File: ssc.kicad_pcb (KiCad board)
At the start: 4 copper layers, 98.8 x 85.1 mm, 25 parts, among them J1 IRQ ENABLE, J2 RS-232 OUT, P1 A2Bus, U1 74HCT245, U2 28C256, U3 1.8432M, U4 SSCGLU, U5 W65C51NxP, U6 MAX3232, U7 MAX3232

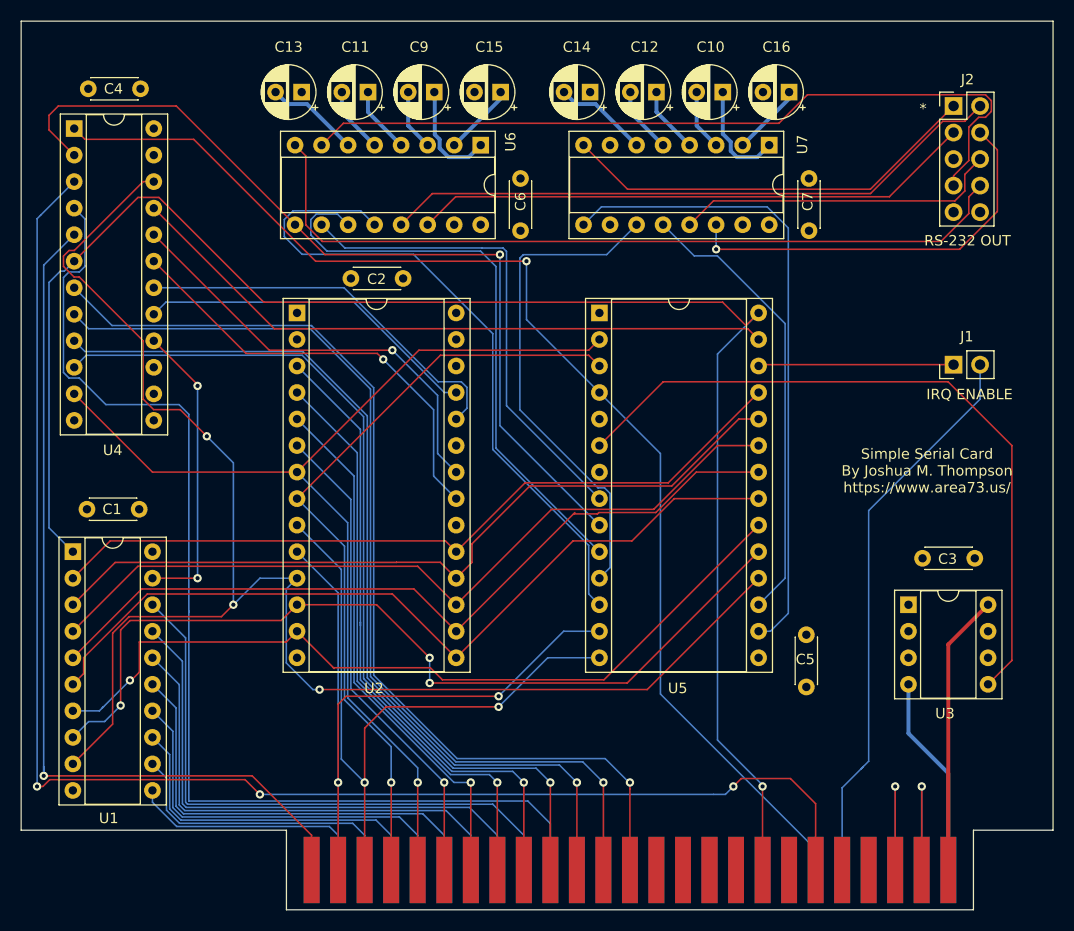
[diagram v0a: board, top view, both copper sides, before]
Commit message: Checkpoint.
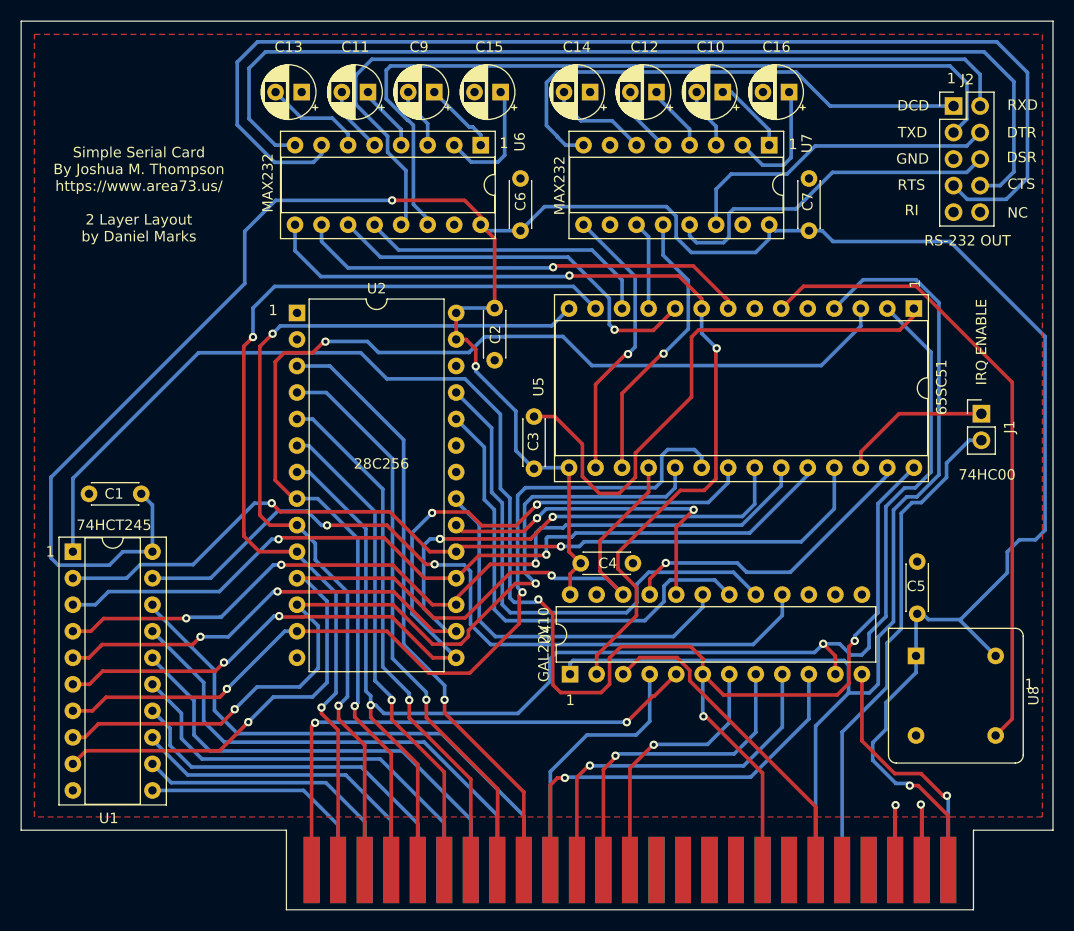
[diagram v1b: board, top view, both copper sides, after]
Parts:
- removed U3: 1.8432M, Package_DIP:DIP-8_W7.62mm_Socket
- added U8: 1.8432M, Oscillator:Oscillator_DIP-8, F.Cu at (187.3, 102.7)
- U1: value 74HCT245 -> 74LS245
- U2: value 28C256 -> 27C256; footprint Package_DIP:DIP-28_W15.24mm_Socket -> Package_DIP:DIP-28_W15.24mm
- U4: footprint Package_DIP:DIP-24_W7.62mm_Socket -> Package_DIP:DIP-24_W7.62mm
- moved U4 70.6 mm to (154.2, 104.4), turned to 90 degrees
- moved C4 62.0 mm to (155.2, 93.8), turned to 0 degrees
- moved C3 43.1 mm to (150.7, 84.8), turned to 90 degrees
- moved U5 30.1 mm to (187.1, 69.4), turned to -90 degrees
- moved C5 12.7 mm to (187.4, 98.7)
- moved C2 9.21 mm to (146.9, 69.4), turned to -90 degrees
- moved J1 5.40 mm to (193.5, 79.5), turned to 0 degrees
- moved C1 1.49 mm to (113.1, 87.2)
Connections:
- net R~W renamed R~{W}
- net ~DEVSEL renamed ~{DEVSEL}
- net ~IOSEL renamed ~{IOSEL}
- net ~IOSTRB renamed ~{IOSTRB}
- net ~IRQ renamed ~{IRQ}
- net ~LATCHCE renamed ~{LATCHCE}
- net ~RES renamed ~{RES}
- J2 pad 9: (no net) -> unconnected-(J2-RI-Pad9)
- P1 pad 14: (no net) -> unconnected-(P1-A12-Pad14)
- P1 pad 15: (no net) -> unconnected-(P1-A13-Pad15)
- P1 pad 16: (no net) -> unconnected-(P1-A14-Pad16)
- P1 pad 17: (no net) -> unconnected-(P1-A15-Pad17)
- P1 pad 19: (no net) -> unconnected-(P1-SYNC-Pad19)
- P1 pad 21: (no net) -> unconnected-(P1-~{RDY}-Pad21)
- P1 pad 22: (no net) -> unconnected-(P1-~{DMA}-Pad22)
- P1 pad 29: (no net) -> unconnected-(P1-~{NMI}-Pad29)
- P1 pad 32: (no net) -> unconnected-(P1-~{INH}-Pad32)
- P1 pad 33: (no net) -> unconnected-(P1--12V-Pad33)
- P1 pad 34: (no net) -> unconnected-(P1--5V-Pad34)
- P1 pad 35: (no net) -> unconnected-(P1-COLORREF/M2B0-Pad35)
- P1 pad 36: (no net) -> unconnected-(P1-7M-Pad36)
- P1 pad 37: (no net) -> unconnected-(P1-Q3-Pad37)
- P1 pad 38: (no net) -> unconnected-(P1-PHI1-Pad38)
- P1 pad 39: (no net) -> unconnected-(P1-USER1/SYNC/M2SEL-Pad39)
- P1 pad 40: (no net) -> unconnected-(P1-PHI0-Pad40)
- P1 pad 50: (no net) -> unconnected-(P1-+12V-Pad50)
- U2 pad 20: GND -> ~{ROMOE}
- U2 pad 22: ~ROMOE -> GND
- U4 pad 20: ~ROMOE -> ~{ROMOE}
- U5 pad 5: (no net) -> unconnected-(U5-RxC-Pad5)
- U5 pad 7: (no net) -> unconnected-(U5-XTAL2-Pad7)
- U7 pad 7: (no net) -> unconnected-(U7-T2OUT-Pad7)
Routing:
- net +5V: track 27.0 -> 262.9 mm, vias 0 -> 3
- net ~{IOSTRB}: track 142.8 -> 31.6 mm, vias 3 -> 0
- net ~{DEVSEL}: track 108.4 -> 25.4 mm
- net A11: track 97.3 -> 25.7 mm
- net A10: track 93.7 -> 31.3 mm
- net GND: track 19.4 -> 77.6 mm, vias 0 -> 1
- net D0: track 146.7 -> 89.6 mm, vias 3 -> 2
- net A9: track 88.7 -> 35.6 mm
- net A8: track 86.1 -> 39.8 mm
- net ~{LATCHCE}: track 28.8 -> 74.4 mm
- net A2: track 74.4 -> 116.9 mm, vias 1 -> 2
- net ~ROMOE: track 41.6 -> 0.00 mm, vias 1 -> 0
- net Net-(U5-~{DTR}): track 47.5 -> 8.50 mm
- net Net-(J2-RTS): track 76.4 -> 113.0 mm
- net Net-(U5-RxD): track 65.2 -> 28.6 mm
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- added copper zone on F.Cu, net GND
- removed copper zone on In1.Cu, net +5V
- removed copper zone on In2.Cu, net GND
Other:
- copper layers 4 -> 2
- net class Default removed
- net class Power removed
- board text added: "1"
- board text added: "28C256"
- board text added: "65SC51"
- board text added: "74HC00"
- board text added: "74HCT245"
- board text added: "CTS"
- board text added: "DCD"
- board text added: "DSR"
- board text added: "DTR"
- board text added: "GAL22V10"
- board text added: "GND"
- board text added: "MAX232"
- board text added: "NC"
- board text added: "RI"
- board text added: "RTS"
- board text added: "RXD"
- board text added: "Simple Serial Card By Joshua M. Thompson https://www.area73.us/ 2 Layer Layout by Daniel Marks"
- board text added: "TXD"
- board text removed: "*"
- board text removed: "Simple Serial Card By Joshua M. Thompson https://www.area73.us/"
